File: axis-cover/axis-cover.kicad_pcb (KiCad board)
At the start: 2 copper layers, 66 x 18 mm, 7 parts

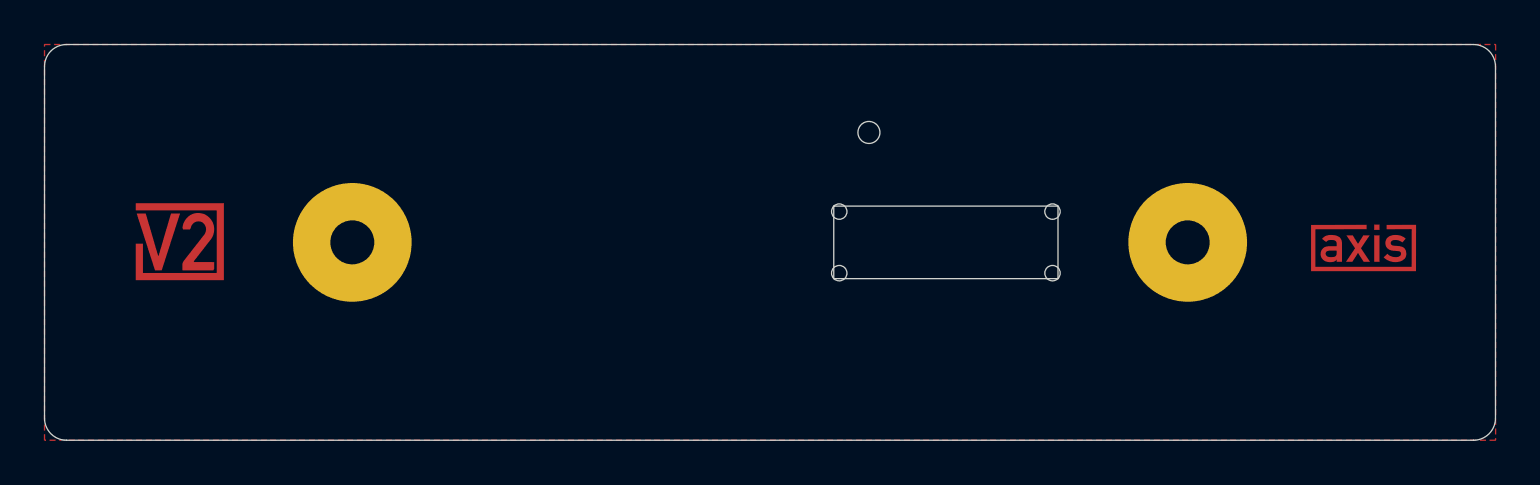
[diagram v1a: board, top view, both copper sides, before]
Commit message: Update
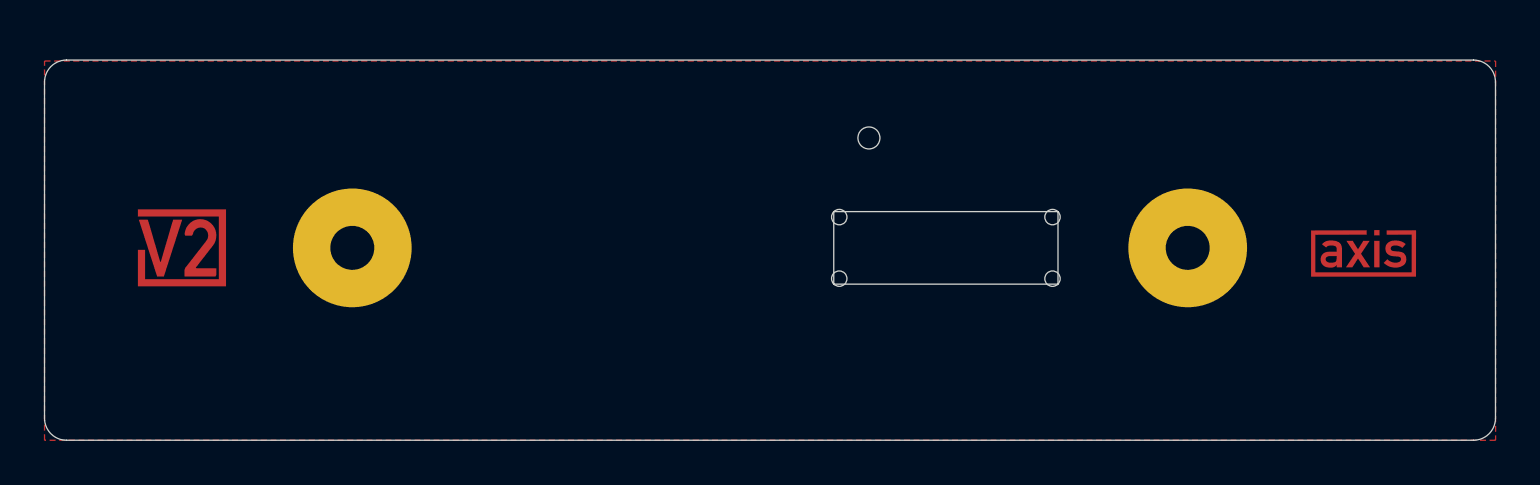
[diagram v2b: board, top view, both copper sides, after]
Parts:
- H2, H3: footprint V2_Mechanical:Mounting_Hole_2mm_Pad_5.2mm -> V2_Mechanical:MountingHole_2mm_Pad_5.2mm
- moved H1 0.25 mm to (154.5, 101.2)
- moved H2 0.25 mm to (169.0, 106.2)
- moved H3 0.25 mm to (131.0, 106.2)
- moved ICON1 0.25 mm to (123.2, 106.2)
- moved ICON2 0.25 mm to (177.0, 106.5)
- moved INFO1 0.25 mm to (150.0, 111.5)
- moved SWT1 0.25 mm to (158.0, 106.2)
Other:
- board size 66 x 18 mm -> 66 x 17.3 mm
